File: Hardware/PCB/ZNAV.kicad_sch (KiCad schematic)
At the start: 11 parts, among them J2 Micro_SD_Card, J3 Display Socket, SW3 RST, SW4 BOOT, U2 NEO-M8N-0, U3 ESP32-S3-WROOM-1

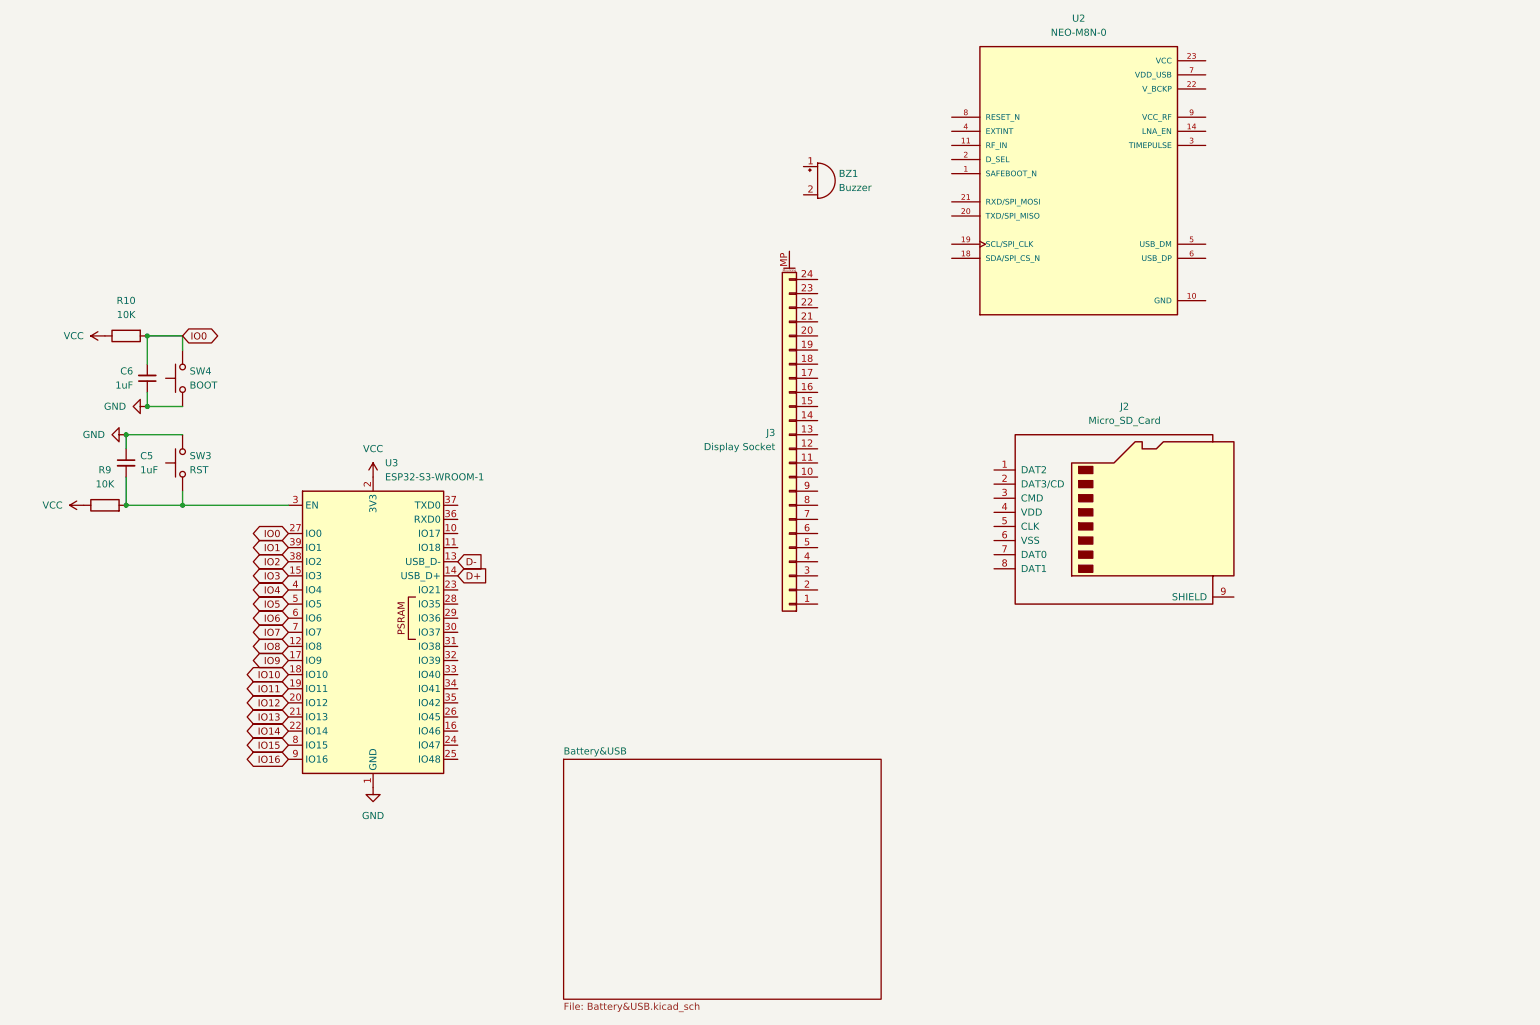
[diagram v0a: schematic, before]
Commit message: updated schematic
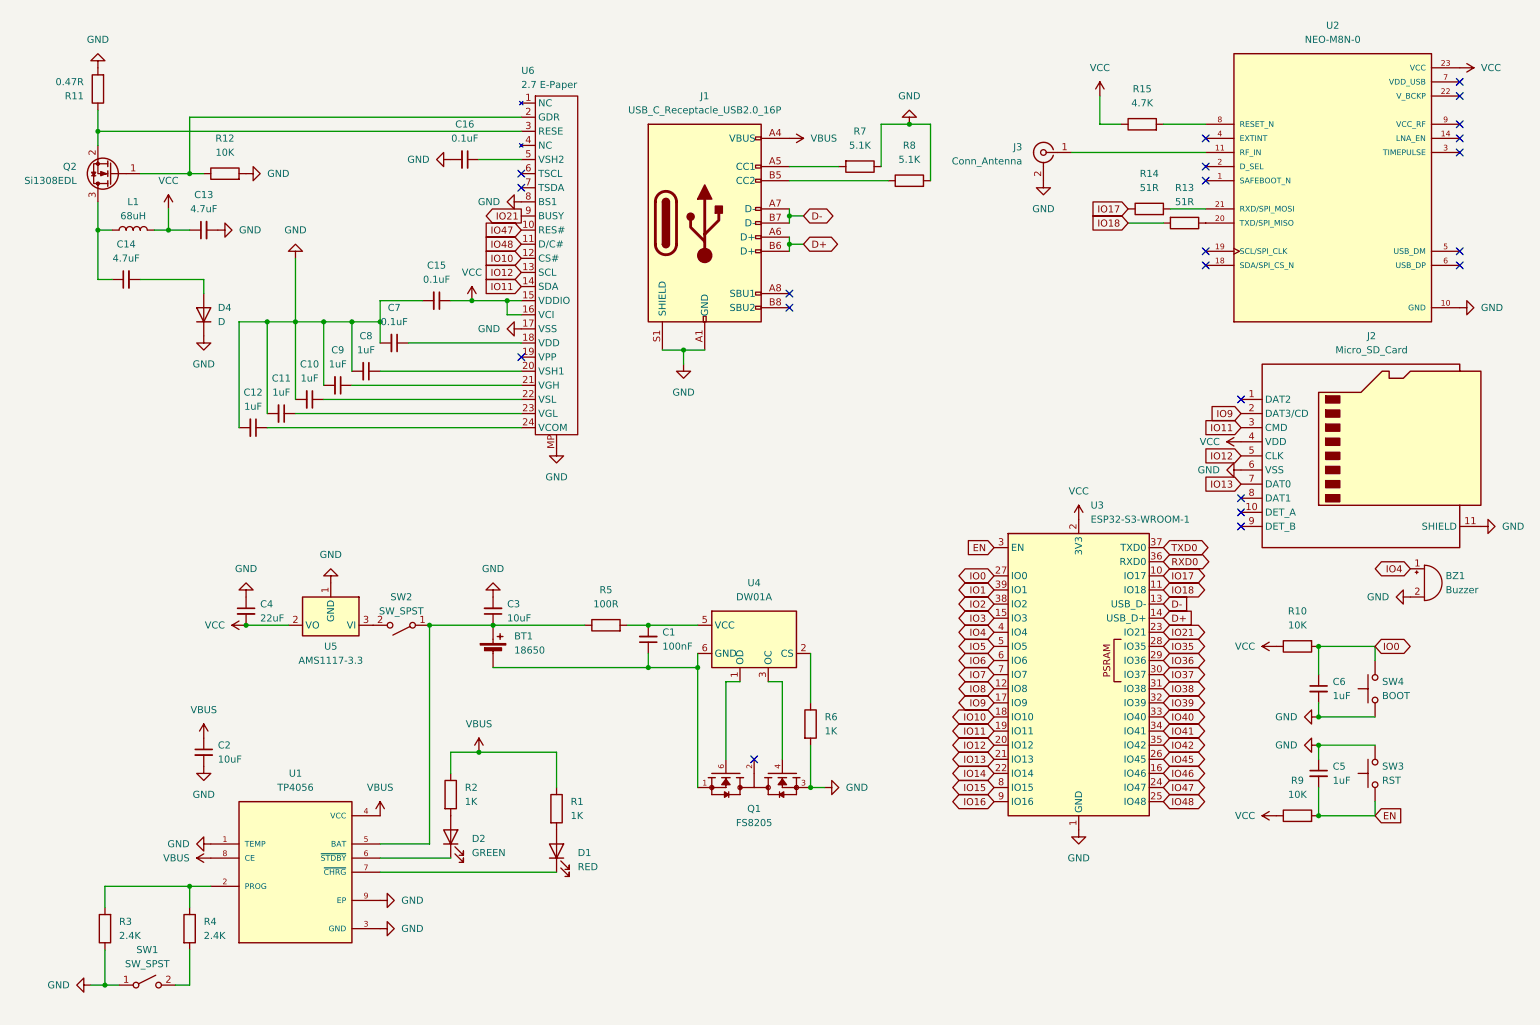
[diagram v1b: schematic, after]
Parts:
- removed J2: Micro_SD_Card, symbol Connector:Micro_SD_Card
- removed J3: Display Socket, symbol Connector_Generic_MountingPin:Conn_01x24_MountingPin
- added BT1: 18650, Battery:BatteryHolder_Keystone_1042_1x18650, symbol Device:Battery_Cell
- added C1: 100nF, Capacitor_SMD:C_0805_2012Metric, symbol Device:C_Small
- added C10, C11, C12, C8, C9: 1uF, Capacitor_SMD:C_0805_2012Metric, symbol Device:C_Small
- added C13, C14: 4.7uF, Capacitor_SMD:C_0805_2012Metric, symbol Device:C_Small
- added C15, C16, C7: 0.1uF, Capacitor_SMD:C_0805_2012Metric, symbol Device:C_Small
- added C2, C3: 10uF, Capacitor_SMD:C_0805_2012Metric, symbol Device:C_Small
- added C4: 22uF, Capacitor_SMD:C_0805_2012Metric, symbol Device:C_Small
- added D1: RED, LED_SMD:LED_0805_2012Metric, symbol Device:LED
- added D2: GREEN, LED_SMD:LED_0805_2012Metric, symbol Device:LED
- added D4: D, Diode_SMD:D_0805_2012Metric, symbol Device:D
- added J1: USB_C_Receptacle_USB2.0_16P, Connector_USB:USB_C_Receptacle_GCT_USB4105-xx-A_16P_TopMnt_Horizontal, symbol Connector:USB_C_Receptacle_USB2.0_16P
- added J2: Micro_SD_Card, Connector_Card:microSD_HC_Hirose_DM3AT-SF-PEJM5, symbol Connector:Micro_SD_Card_Det_Hirose_DM3AT
- added J3: Conn_Antenna, RF_Antenna:Astrocast_AST50127-00, symbol Connector:Conn_Coaxial
- added L1: 68uH, Inductor_SMD:L_0805_2012Metric, symbol Device:L
- added Q1: FS8205, FS8205:SOT95P280X145-6N, symbol FS8205:FS8205
- added Q2: Si1308EDL, Package_TO_SOT_SMD:SOT-323_SC-70, symbol Transistor_FET:Si1308EDL
- added R1, R2, R6: 1K, Resistor_SMD:R_0805_2012Metric, symbol Device:R
- added R11: 0.47R, Resistor_SMD:R_0805_2012Metric, symbol Device:R
- added R12: 10K, Resistor_SMD:R_0805_2012Metric, symbol Device:R
- added R13, R14: 51R, Resistor_SMD:R_0805_2012Metric, symbol Device:R
- added R15: 4.7K, Resistor_SMD:R_0805_2012Metric, symbol Device:R
- added R3, R4: 2.4K, Resistor_SMD:R_0805_2012Metric, symbol Device:R
- added R5: 100R, Resistor_SMD:R_0805_2012Metric, symbol Device:R
- added R7, R8: 5.1K, Resistor_SMD:R_0805_2012Metric, symbol Device:R
- added SW1, SW2: SW_SPST, Button_Switch_THT:SW_DIP_SPSTx01_Slide_6.7x4.1mm_W7.62mm_P2.54mm_LowProfile, symbol Switch:SW_SPST
- added U1: TP4056, TP4056:SOP127P600X175-9N, symbol TP4056:TP4056
- added U4: DW01A, Package_TO_SOT_SMD:SOT-23-6, symbol Battery_Management:DW01A
- added U5: AMS1117-3.3, Package_TO_SOT_SMD:SOT-223-3_TabPin2, symbol Regulator_Linear:AMS1117-3.3
- added U6: 2.7 E-Paper, Connector_FFC-FPC:Hirose_FH12-24S-0.5SH_1x24-1MP_P0.50mm_Horizontal, symbol MyLib:2.7_epaper
- BZ1: footprint (none) -> Buzzer_Beeper:Buzzer_12x9.5RM7.6
- C5, C6: footprint (none) -> Capacitor_SMD:C_0805_2012Metric
- R10, R9: footprint (none) -> Resistor_SMD:R_0805_2012Metric
- SW3, SW4: footprint (none) -> Button_Switch_THT:SW_PUSH_6mm_H5mm
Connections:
- net D+: now also J1.A6 (D+), J1.B6 (D+)
- net D-: now also J1.A7 (D-), J1.B7 (D-)
- net GND: now also BZ1.2 (-), C6.2, C10.2, C11.2, C12.2, C13.2, C15.2, C16.2, C2.2, C3.2, C4.1, C7.2, C8.2, C9.2, D4.1 (K), J1.A1 (GND), J1.A12 (GND), J1.B1 (GND), J1.B12 (GND), J1.S1 (SHIELD), J2.11 (SHIELD), J2.6 (VSS), J3.2 (Ext), Q1.3, R11.2, R12.2, R3.1, R6.2, R7.1, R8.2, SW1.1 (A), U1.1 (TEMP), U1.3 (GND), U1.9 (EP), U5.1 (GND), U6.17 (VSS), U6.8 (BS1), U6.MP; no longer C6.1
- net IO0: now also C6.1; no longer C6.2
- net IO10: now also U6.12 (CS#)
- net IO11: now also J2.3 (CMD), U6.14 (SDA)
- net IO12: now also J2.5 (CLK), U6.13 (SCL)
- net IO13: now also J2.7 (DAT0)
- net IO4: now also BZ1.1 (+)
- net IO9: now also J2.2 (DAT3/CD)
- net VCC: now also U2.23 (VCC), C13.1, C15.1, C4.2, J2.4 (VDD), L1.2, R15.1, U5.2 (VO), U6.15 (VDDIO), U6.16 (VCI)
- net EN: now reaches C5.2, R9.2, SW3.1, U3.3 (EN)
- net IO17: now reaches U3.10 (IO17)
- net IO17: now also R14.1
- net IO18: now reaches U3.11 (IO18)
- net IO18: now also R13.2
- net IO46: now reaches U3.16 (IO46)
- net IO21: now reaches U3.23 (IO21)
- net IO21: now also U6.9 (BUSY)
- net IO47: now reaches U3.24 (IO47)
- net IO47: now also U6.10 (RES#)
- net IO48: now reaches U3.25 (IO48)
- net IO48: now also U6.11 (D/C#)
- net IO45: now reaches U3.26 (IO45)
- net IO35: now reaches U3.28 (IO35)
- net IO36: now reaches U3.29 (IO36)
- net IO37: now reaches U3.30 (IO37)
- net IO38: now reaches U3.31 (IO38)
- net IO39: now reaches U3.32 (IO39)
- net IO40: now reaches U3.33 (IO40)
- net IO41: now reaches U3.34 (IO41)
- net IO42: now reaches U3.35 (IO42)
- net RXD0: now reaches U3.36 (RXD0)
- net TXD0: now reaches U3.37 (TXD0)
- net at U2.11 (RF_IN): now also J3.1 (In)
- net at U2.20 (TXD/SPI_MISO): now also R13.1
- net at U2.21 (RXD/SPI_MOSI): now also R14.2
- net at U2.8 (RESET_N): now also R15.2
- new net: C14.1, L1.1, Q2.3 (D)
- new net: C14.2, D4.2 (A)
- new net: C7.1, U6.18 (VDD)
- new net: BT1.1 (+), C3.1, R5.1, SW2.1 (A), U1.5 (BAT)
- new net: SW2.2 (B), U5.3 (VI)
- new net: Q2.1 (G), R12.1, U6.2 (GDR)
- new net: C8.1, U6.20 (VSH1)
- new net: C9.1, U6.21 (VGH)
- new net: C10.1, U6.22 (VSL)
- new net: C11.1, U6.23 (VGL)
- new net: C12.1, U6.24 (VCOM)
- new net: Q2.2 (S), R11.1, U6.3 (RESE)
- new net: C16.1, U6.5 (VSH2)
- new net: R3.2, R4.1, U1.2 (PROG)
- new net: D2.1 (K), U1.6 (~{STDBY})
- new net: D1.1 (K), U1.7 (~{CHRG})
- new net: J1.B5 (CC2), R8.1
- new net: Q1.6, U4.1 (OD)
- new net: R6.1, U4.2 (CS)
- new net: Q1.4, U4.3 (OC)
- new net: C1.2, R5.2, U4.5 (VCC)
- new net: BT1.2 (-), C1.1, Q1.1, U4.6 (GND)
- new net: D1.2 (A), R1.2
- new net: D2.2 (A), R2.2
- new net: J1.A5 (CC1), R7.2
- new net: Q1.2, Q1.5
- new net: R4.2, SW1.2 (B)
- new net VBUS: C2.1, J1.A4 (VBUS), J1.A9 (VBUS), J1.B4 (VBUS), J1.B9 (VBUS), R1.1, R2.1, U1.4 (VCC), U1.8 (CE)
- no-connect marks 0 -> 22
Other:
- removed sheet Battery&USB
- moved on the sheet: BZ1, C5, C6, R10, R9, SW3, SW4, U2, U3
